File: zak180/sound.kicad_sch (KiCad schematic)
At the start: 19 parts, among them J4 Speaker, U11 74HC02, U16 74HC00, U17 LM386, U3 PSG_AY-3-8912

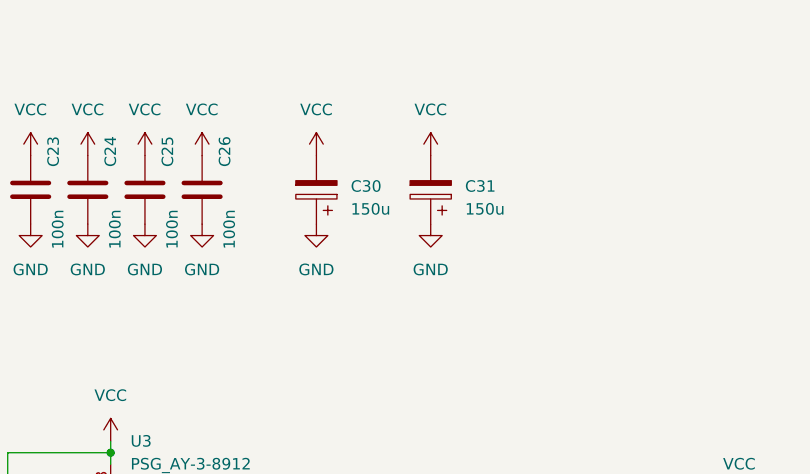
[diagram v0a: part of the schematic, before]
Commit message: HW: PCB complete
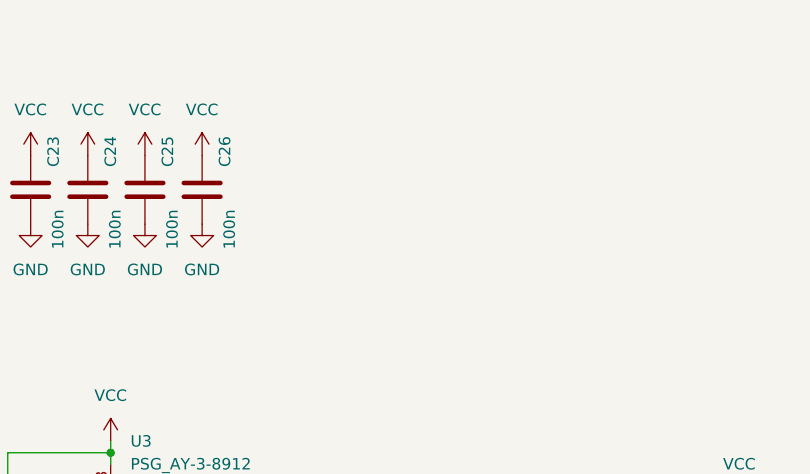
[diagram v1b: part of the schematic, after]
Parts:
- removed C30, C31: 150u, Capacitor_THT:CP_Radial_D10.0mm_P5.00mm, symbol Device:C_Polarized
- J4: footprint Connector_PinHeader_1.00mm:PinHeader_1x02_P1.00mm_Vertical -> Connector_PinHeader_2.54mm:PinHeader_1x02_P2.54mm_Horizontal
